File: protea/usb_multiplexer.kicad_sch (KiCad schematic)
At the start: 3 parts, among them U10 TS3USB221RSER

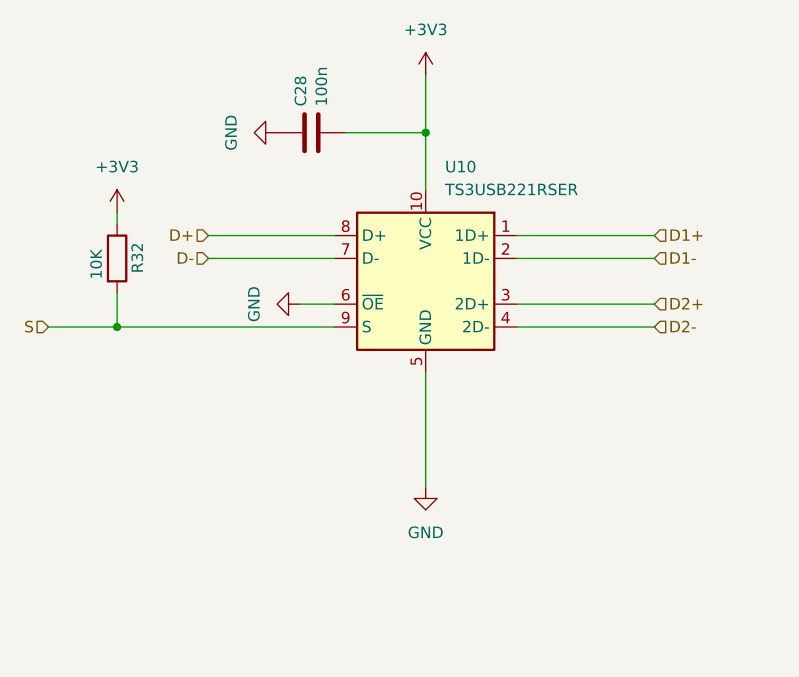
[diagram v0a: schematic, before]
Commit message: Protea HW 2.06
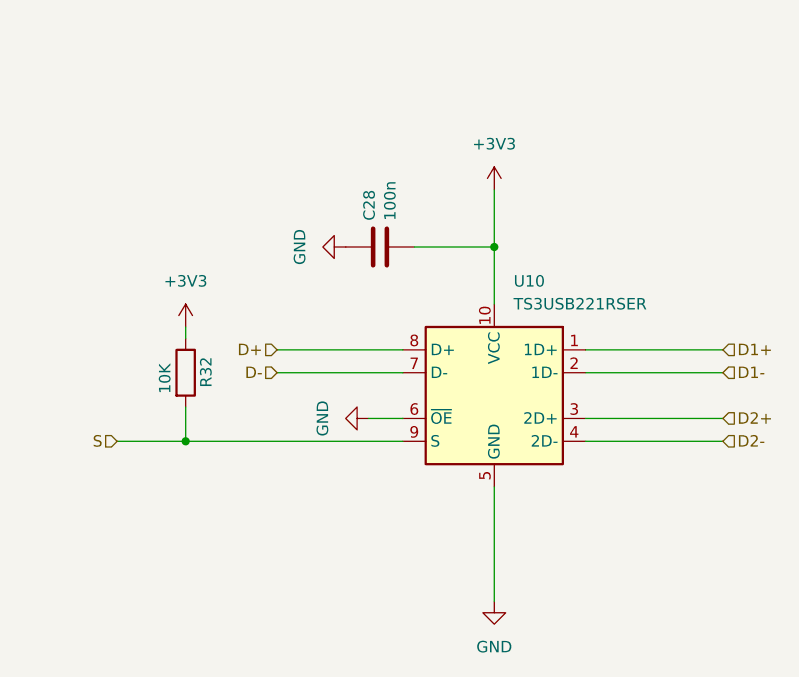
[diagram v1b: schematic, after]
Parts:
- U10: AliExpress (none) -> https://vi.aliexpress.com/item/1005004217168769.html
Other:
- moved on the sheet: C28, R32, U10
